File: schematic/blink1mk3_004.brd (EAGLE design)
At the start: 88.5 x 50.8 mm, 36 parts, among them J1 NONPOP, U1 EFM32HG309F64G, X1 USBPCB2, X2 USBPCB2, X3 USBPCB2

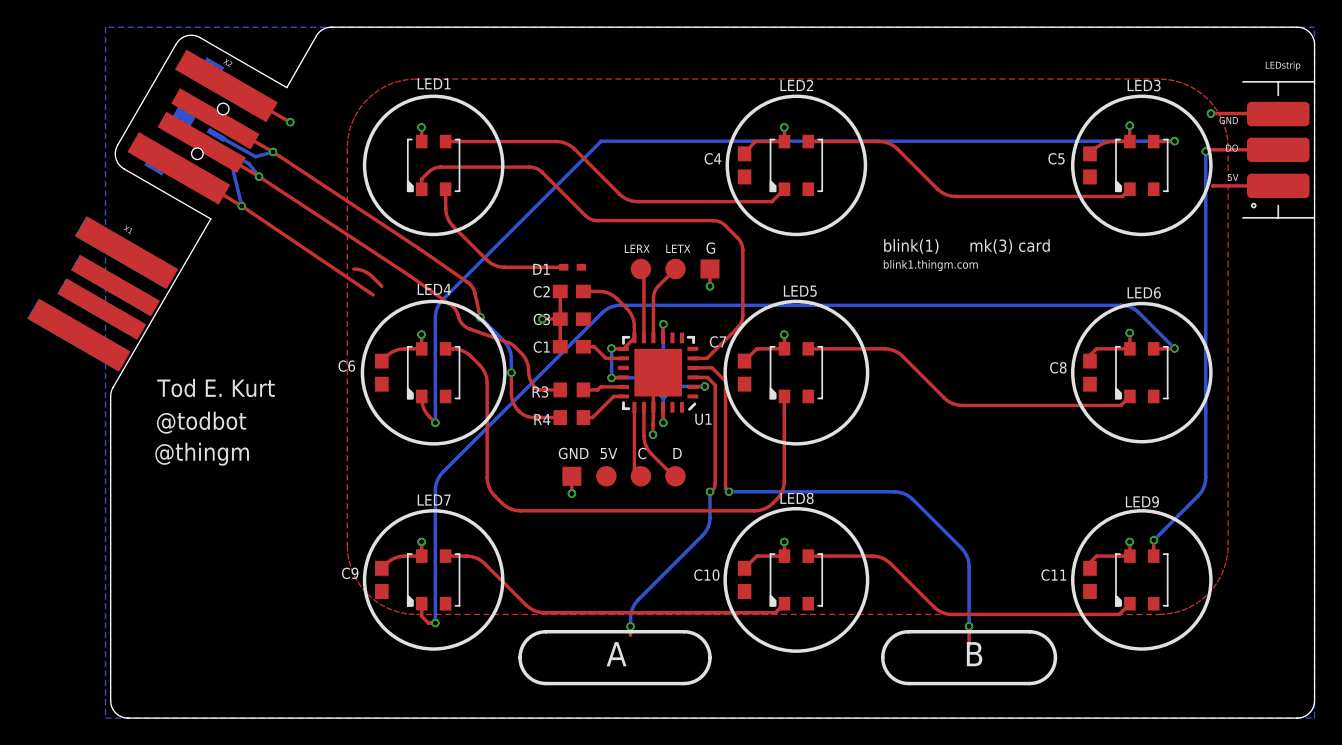
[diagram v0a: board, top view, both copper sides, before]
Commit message: sync schematic experiments
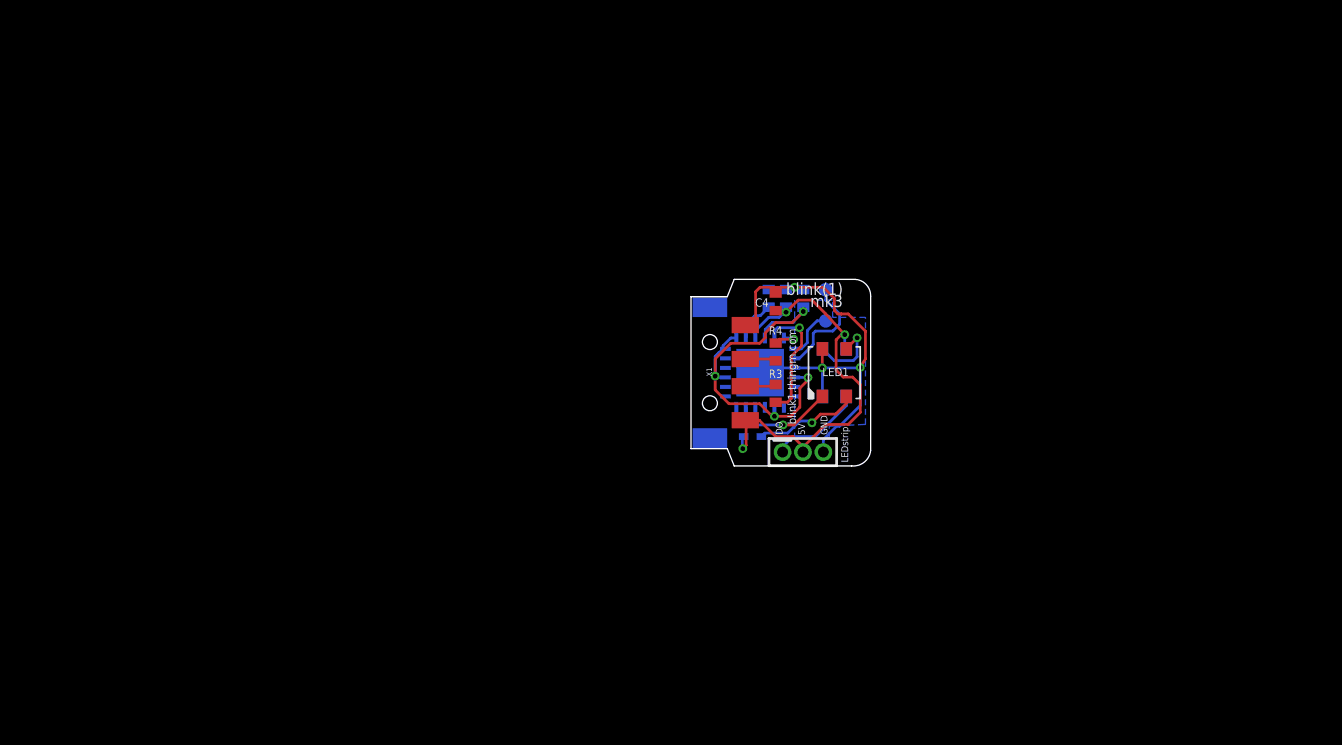
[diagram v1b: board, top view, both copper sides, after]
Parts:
- removed 5V, LERX, LETX: TPTP15R, testpad:TP15R
- removed C10, C11, C5, C6, C7, C8, C9: 0.1uF, adafruit:C0603
- removed G, GND: TPTP14SQ, testpad:TP14SQ
- removed J1: NONPOP, SparkFun-Connectors:USB-B-MICRO-SMD
- removed LED3, LED4, LED5, LED6, LED7, LED8, LED9: SK6812MINI, adafruit:LED3535
- removed U$1: LED_STRIP_3P, NeoJoints:LEDSTRIP-3P
- removed X2, X3: USBPCB2, todstuff:USB-A-PCB-2
- added JP3: M03MM, todstuff:1X03-1.5MM
- C, D: value TPTP15R -> TPTP10R; device testpad:TP15R -> testpad:TP10R
- C1, C2, C3, C4: device adafruit:C0603 -> adafruit:C0402
- LED1, LED2: value SK6812MINI -> WS2812B3535
- R3, R4: device adafruit:R0603 -> adafruit:R0402
- X1: value USBPCB2 -> USB; device todstuff:USB-A-PCB-2 -> todstuff:MOLEX-48037-1000
- moved X1 43.6 mm to (-0.01, 0.00), turned to 0 degrees
- moved LED1 33.2 mm to (9.14, 0.00)
- moved D1 18.2 mm to (3.17, -4.70), flipped to the bottom
- moved C 17.8 mm to (8.51, 3.81), flipped to the bottom
- moved D 17.6 mm to (8.51, 6.10), flipped to the bottom
- moved C2 17.0 mm to (6.86, 5.46), flipped to the bottom, turned to 90 degrees
- moved C3 15.8 mm to (5.59, 5.46), flipped to the bottom, turned to 90 degrees
- moved R4 15.7 mm to (4.83, 1.52), turned to 270 degrees
- moved LED2 15.5 mm to (9.14, 0.00), flipped to the bottom, turned to 270 degrees
- moved R3 15.0 mm to (4.83, -1.52), turned to 90 degrees
- moved C1 14.9 mm to (4.32, 5.46), flipped to the bottom, turned to 90 degrees
- moved C4 10.3 mm to (4.83, 5.21)
- moved U1 7.49 mm to (3.68, 0.00), flipped to the bottom, turned to 90 degrees
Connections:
- removed net N$10: LED6.3, LED7.1
- removed net N$4: LED7.3, LED8.1
- removed net N$5: LED4.3, LED5.1
- removed net N$6: LED5.3, LED6.1
- removed net N$7: LED2.3, LED3.1
- removed net N$8: LED3.3, LED4.1
- removed net N$9: LED8.3, LED9.1
- removed net VBUS: X1.5V, X3.5V
- net +5V: now also JP3.2, X1.1; no longer 5V.TP, C10.1, C11.1, C5.1, C6.1, C7.1, C8.1, C9.1, J1.VBUS, LED3.2, LED4.2, LED5.2, LED6.2, LED7.2, LED8.2, LED9.2, U$1.A, X2.5V
- net DO: now also JP3.1, LED2.3; no longer LED9.3, U$1.B
- net GND: now also JP3.3, X1.4; no longer C10.2, C11.2, C5.2, C6.2, C7.2, C8.2, C9.2, G.TP, GND.TP, J1.GND, LED3.4, LED4.4, LED5.4, LED6.4, LED7.4, LED8.4, LED9.4, U$1.C, X1.GND, X2.GND, X3.GND
- net LEUO_RX: no longer LERX.TP
- net LEUO_TX: no longer LETX.TP
- net USB_D+: now also X1.3; no longer J1.D+, X2.USB_P
- net USB_D-: now also X1.2; no longer J1.D-, X2.USB_M
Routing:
- net N$10: track 74.9 -> 0.00 mm, vias 2 -> 0
- net N$8: track 71.7 -> 0.00 mm, vias 2 -> 0
- net N$5: track 41.7 -> 0.00 mm
- net USB_D+: track 40.5 -> 2.77 mm, vias 3 -> 0
- net CAP1A: track 37.0 -> 0.00 mm, vias 2 -> 0
- net USB_D-: track 37.3 -> 2.77 mm, vias 1 -> 0
- net DI: track 37.2 -> 7.39 mm, vias 0 -> 1
- net DO: track 36.6 -> 7.42 mm, vias 2 -> 0
- net N$4: track 26.7 -> 0.00 mm
- net N$9: track 25.5 -> 0.00 mm
- net N$6: track 25.4 -> 0.00 mm
- net N$7: track 25.3 -> 0.00 mm
- net CAP0A: track 22.6 -> 0.00 mm, vias 2 -> 0
- net N$2: track 26.9 -> 5.71 mm, vias 0 -> 1
- net GND: track 59.3 -> 39.5 mm, vias 15 -> 3
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- removed copper zone on layer 1, net +5V
- removed copper zone on layer 1, net CAP0A
- removed copper zone on layer 1, net CAP1A
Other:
- board size 88.5 x 50.8 mm -> 13.2 x 13.7 mm
- board text added: "blink1mk3_002"
- board text added: "mk3"
- board text removed: "@thingm"
- board text removed: "@todbot"
- board text removed: "A"
- board text removed: "B"
- board text removed: "Tod E. Kurt"
- board text removed: "blink1mk3_card"
- board text removed: "mk(3) card"
